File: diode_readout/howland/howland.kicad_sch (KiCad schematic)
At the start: 10 parts, among them J1 Conn_01x04, J2 JST_SH_Conn_01x04_i2c_horizon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, U1 FM24C64C

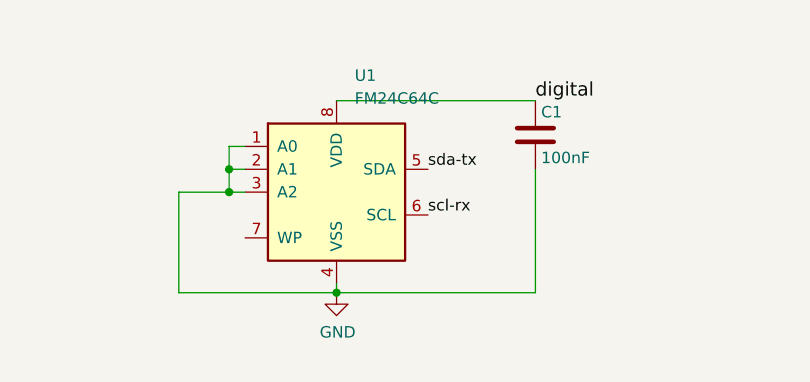
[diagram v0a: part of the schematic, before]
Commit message: Keep boards up to date
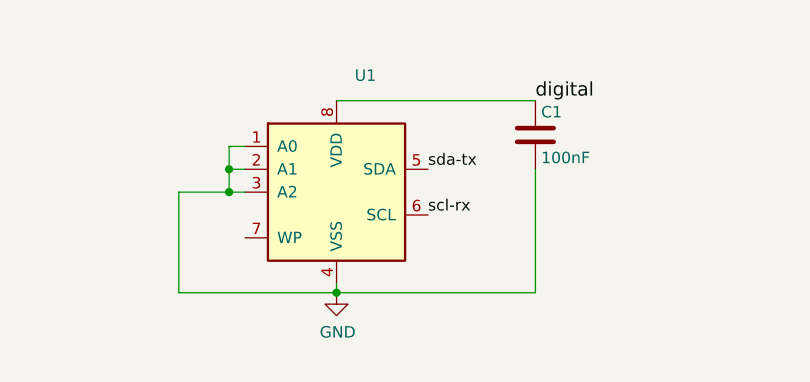
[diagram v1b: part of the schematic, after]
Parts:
- U1: value FM24C64C -> (none); footprint Package_SO:SOIC-8_3.9x4.9mm_P1.27mm -> (none)
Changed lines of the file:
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@@
       (effects (font (size 1.27 1.27)) (justify left))
     )
-    (property "Value" "FM24C64C" (id 1) (at 110.9854 35.56 0)
+    (property "Value" "" (id 1) (at 110.9854 35.56 0)
       (effects (font (size 1.27 1.27)) (justify left))
     )
-    (property "Footprint" "Package_SO:SOIC-8_3.9x4.9mm_P1.27mm" (id 2) (at 108.966 45.974 0)
-      (effects (font (size 1.27 1.27)) hide)
-    )
-    (property "Datasheet" "http://www.cypress.com/file/41651/download" (id 3) (at 103.886 37.084 0)
+    (property "Footprint" "" (id 2) (at 108.966 45.974 0)
+      (effects (font (size 1.27 1.27)) hide)
+    )
+    (property "Datasheet" "https://datasheet.lcsc.com/lcsc/1806121739_Cypress-Semicon-FM24V05-GTR_C66021.pdf" (id 3) (at 103.886 37.084 0)
       (effects (font (size 1.27 1.27)) hide)
     )
@@
     )
     (path "/ab88f3e0-e707-48e0-91f8-7ac28f1ec265"
-      (reference "U1") (unit 1) (value "FM24C64C") (footprint "Package_SO:SOIC-8_3.9x4.9mm_P1.27mm")
+      (reference "U1") (unit 1) (value "FM24V05") (footprint "Package_SO:SOIC-8_3.9x4.9mm_P1.27mm")
     )
     (path "/00000000-0000-0000-0000-000059ed3d7b/e9890516-b047-4c9e-9731-dd57dc45efd4"
